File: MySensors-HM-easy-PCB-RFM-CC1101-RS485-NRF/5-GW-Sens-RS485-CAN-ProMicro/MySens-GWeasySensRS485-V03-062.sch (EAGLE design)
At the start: 27 parts, among them IC1 LM1117MPX-ADJ, IC2 LD117ADT50TR, IC6 LM1117MPX-ADJ, X4 1751264

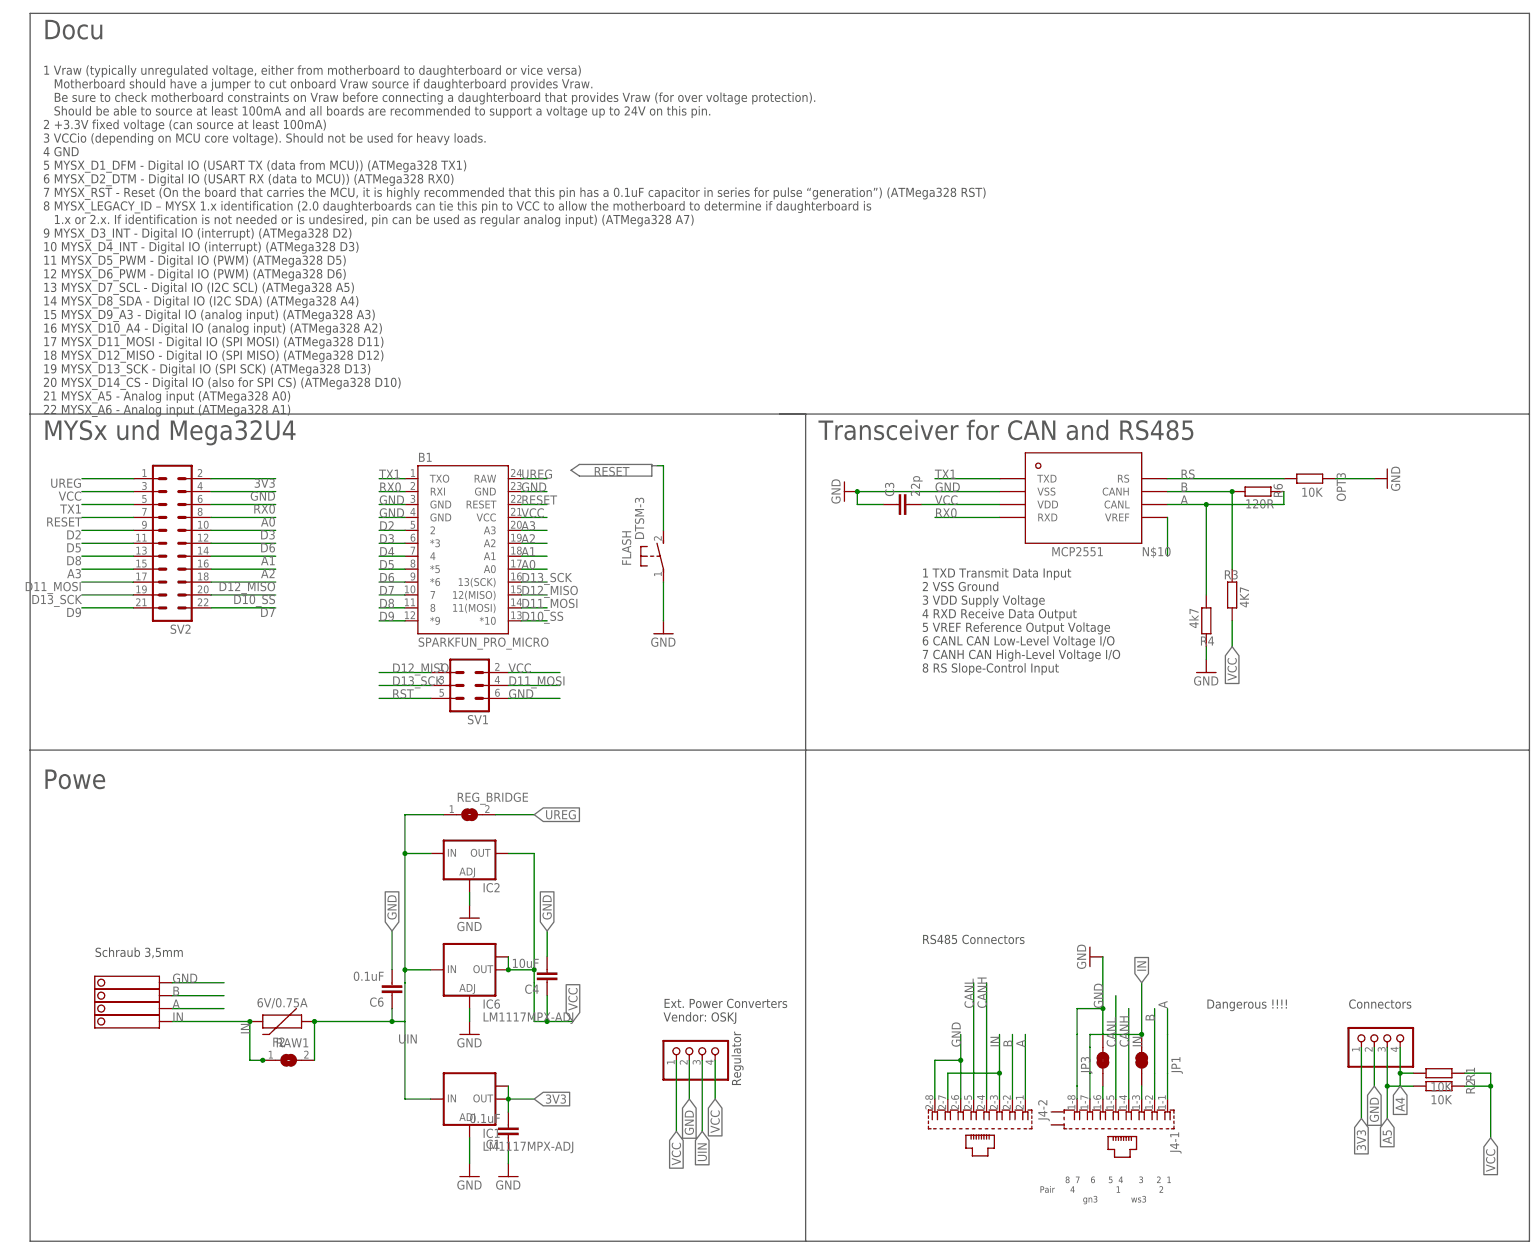
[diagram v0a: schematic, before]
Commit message: div
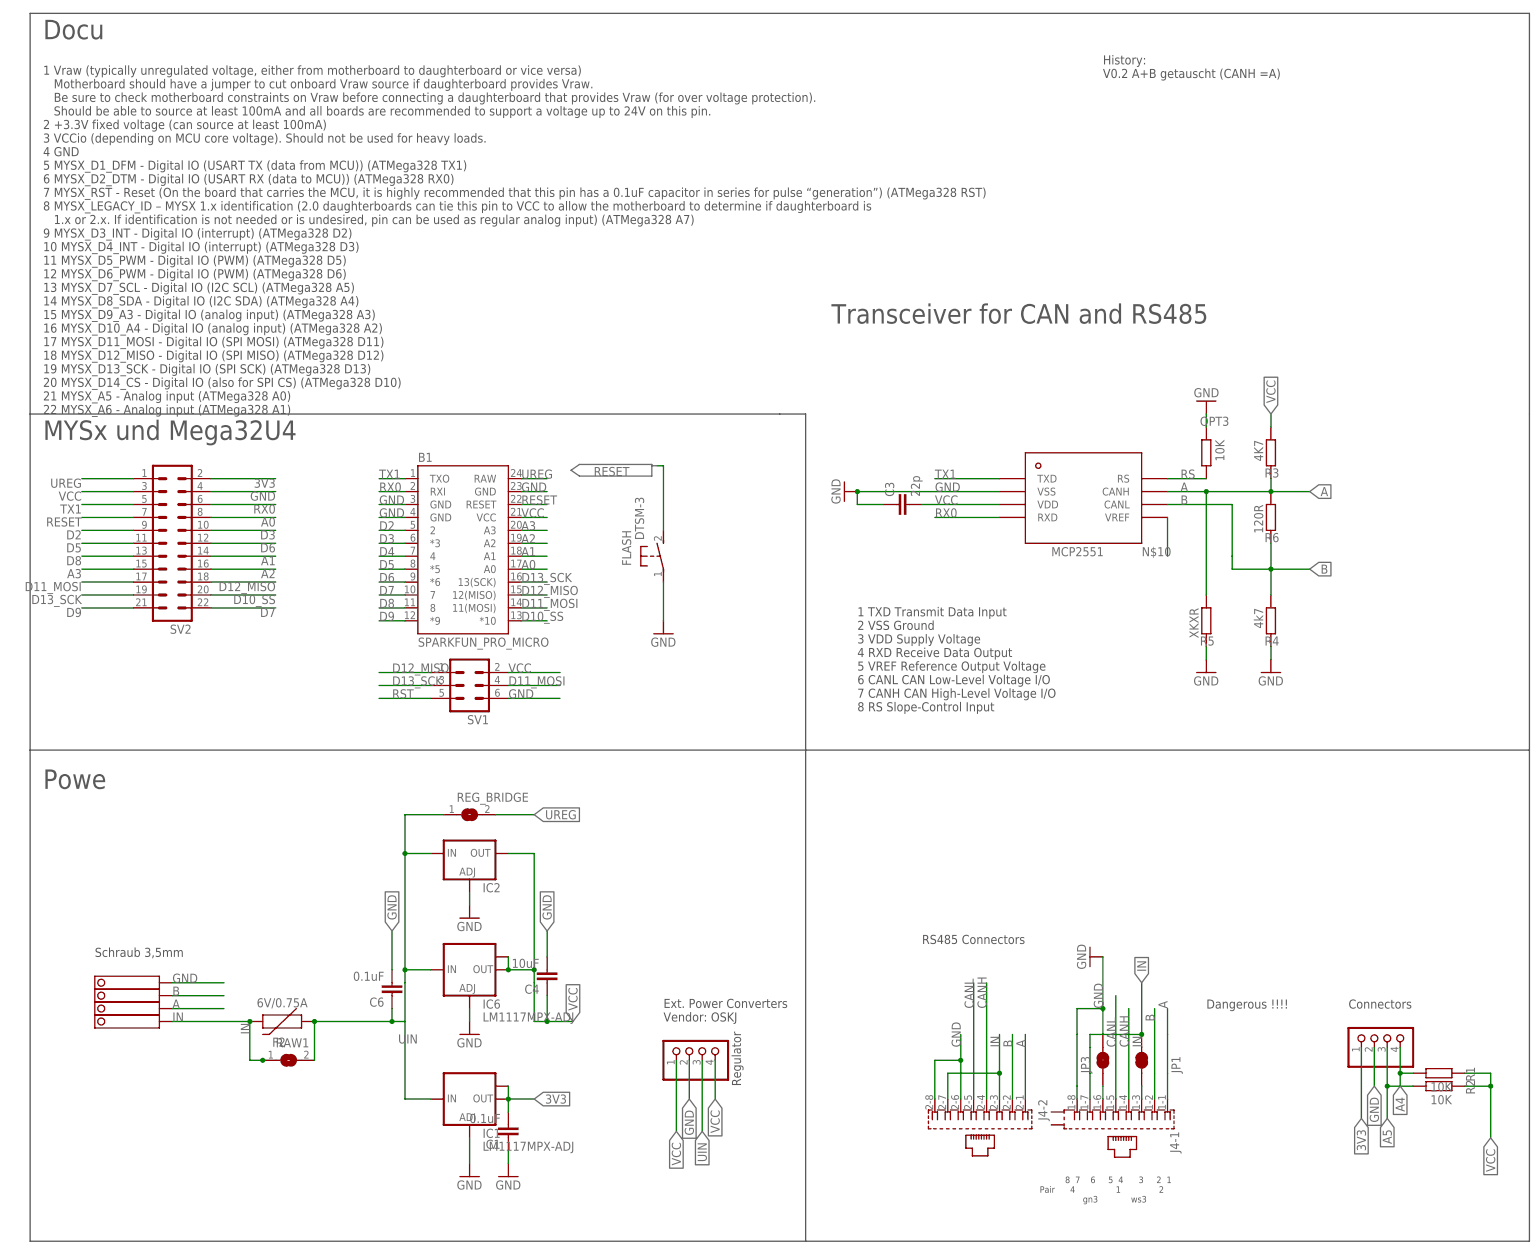
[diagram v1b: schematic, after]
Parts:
- added R5: XKXR, rcl:R-EU_R0805
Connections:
- net A: now also R3.2, R5.1, R6.1, U$1.CANH; no longer R4.1, R6.2, U$1.CANL
- net B: now also R4.1, R6.2, U$1.CANL; no longer R3.2, R6.1, U$1.CANH
- net GND: now also R5.2
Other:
- note added: "History: V0.2 A+B getauscht (CANH =A)"
- moved on the sheet: OPT3, R3, R4, R6
